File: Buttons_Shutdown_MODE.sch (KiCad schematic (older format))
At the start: 7 parts

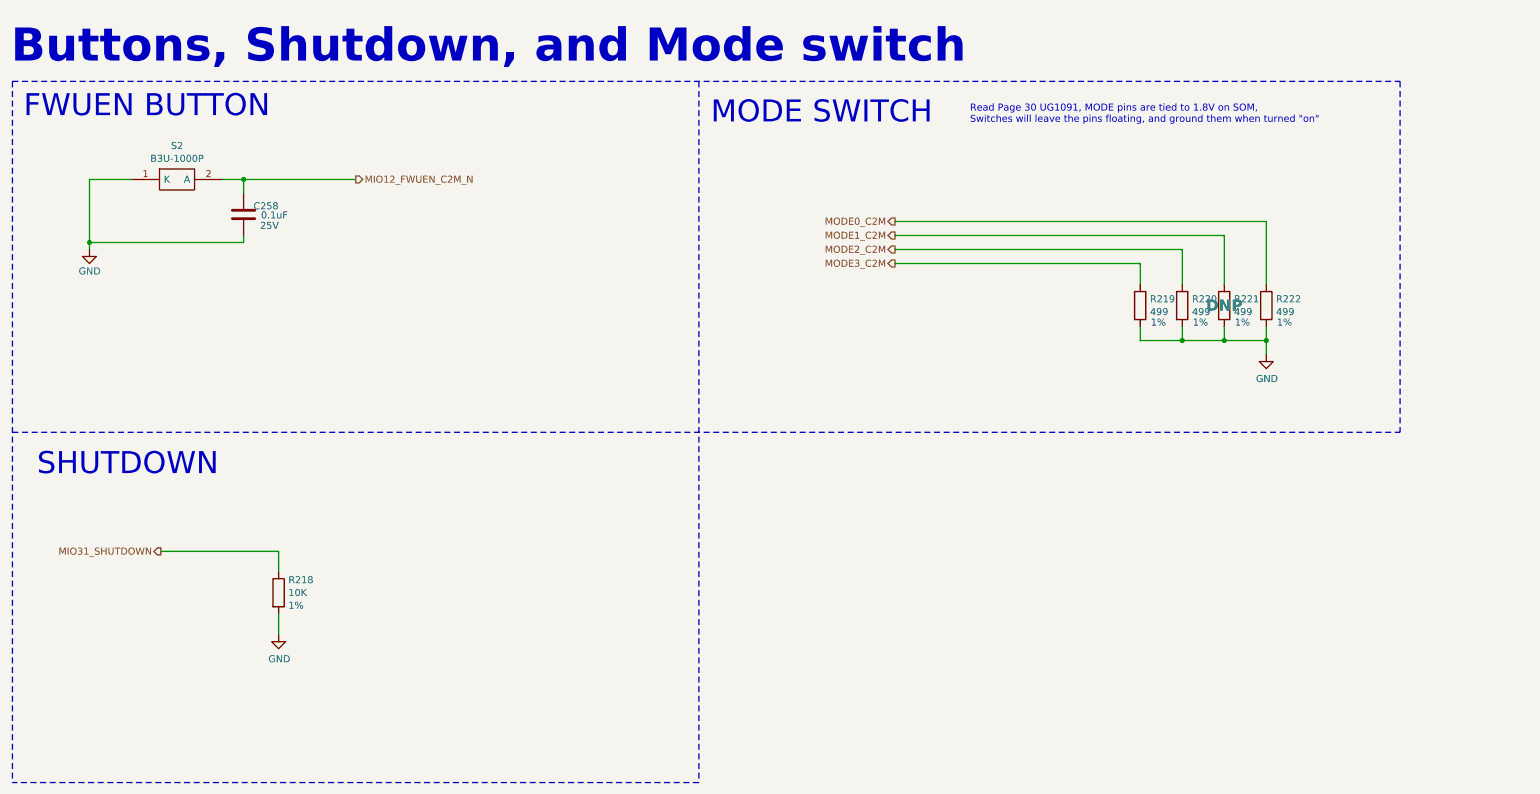
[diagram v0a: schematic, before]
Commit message: Update May --> See Update Note
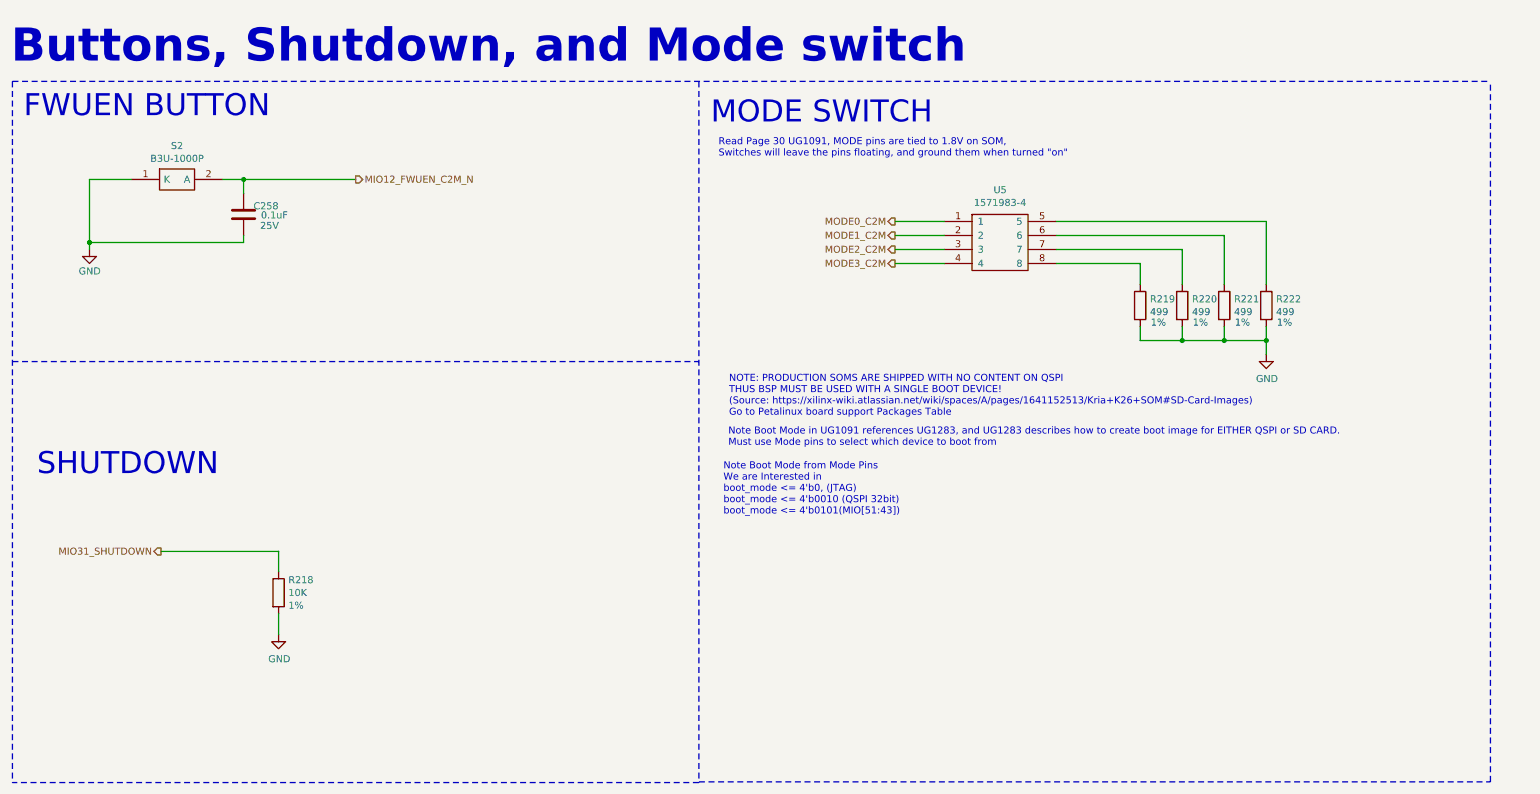
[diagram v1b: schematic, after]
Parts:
- added U5: 1571983-4, ApotheoTech_CXP_Lib:1571983-4, symbol ApotheoTech:1571983-4
- R221: DNP DNP -> (none)
- S2: footprint B3U-1000P -> ApotheoTech_CXP_Lib:B3U-1000P
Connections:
- net MODE0_C2M: now also U5.1; no longer R222.1
- net MODE1_C2M: now also U5.2; no longer R221.1
- net MODE2_C2M: now also U5.3; no longer R220.1
- net MODE3_C2M: now also U5.4; no longer R219.1
- new net: R219.1, U5.8
- new net: R220.1, U5.7
- new net: R221.1, U5.6
- new net: R222.1, U5.5
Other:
- note added: "NOTE: PRODUCTION SOMS ARE SHIPPED WITH NO CONTENT ON QSPI\nTHUS BSP MUST BE USED WITH A SINGLE BOOT DEVICE! \n(Source: https://xilinx-wiki.atlassian.net/wiki/spaces/A/pages/1641152513/Kria+K26+SOM#SD-Card-Images)\nGo to Petalinux board support Packages Table"
- note added: "Note Boot Mode from Mode Pins\nWe are Interested in \nboot_mode <= 4'b0, (JTAG)\nboot_mode <= 4'b0010 (QSPI 32bit)\nboot_mode <= 4'b0101(MIO[51:43])\n"
- note added: "Note Boot Mode in UG1091 references UG1283, and UG1283 describes how to create boot image for EITHER QSPI or SD CARD.\nMust use Mode pins to select which device to boot from\n"
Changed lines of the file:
@@
 F 0 "S2" H 1775 1940 50  0000 C CNN
 F 1 "B3U-1000P" H 1775 1849 50  0000 C CNN
-F 2 "B3U-1000P" H 2425 1800 50  0001 L CNN
+F 2 "ApotheoTech_CXP_Lib:B3U-1000P" H 2425 1800 50  0001 L CNN
 F 3 "https://www.omron.com/ecb/products/pdf/en-b3u.pdf" H 2425 1700 50  0001 L CNN
 F 4 "OMRON ELECTRONIC COMPONENTS - B3U-1000P - SWITCH, SPST-NO, 0.05A, 12V, SMD" H 2425 1600 50  0001 L CNN "Description"
@@
 Text HLabel 3050 1700 2    50   Output ~ 0
 MIO12_FWUEN_C2M_N
-Wire Notes Line
-	10505 1000 10505 3505
-Wire Notes Line
-	600  1000 10505 1000
-Wire Notes Line
-	600  3505 10505 3505
 Text Notes 5585 1315 0    157  ~ 0
 MODE SWITCH
 Text Notes 775  3825 0    157  ~ 0
 SHUTDOWN
-Text Notes 7435 1305 0    50   ~ 0
+Text Notes 5640 1545 0    50   ~ 0
 Read Page 30 UG1091, MODE pins are tied to 1.8V on SOM,\nSwitches will leave the pins floating, and ground them when turned "on"
 Text HLabel 6900 2000 0    50   Output ~ 0
@@
 F 5 "1%" H 9380 2480 50  0000 C CNN "Tol"
 F 6 "1/10W" H 9250 2600 50  0001 C CNN "Power"
-F 7 "DNP" H 9250 2600 79  0000 C CNB "DNP"
 	1    9250 2600
 	1    0    0    -1
@@
 Wire Notes Line
 	600  1000 600  6005
-Wire Wire Line
-	6900 2000 9550 2000
-Wire Wire Line
-	6900 2100 9250 2100
-Wire Wire Line
-	6900 2200 8950 2200
-Wire Wire Line
-	6900 2300 8650 2300
 $Comp
 L Device:R R?
@@
 	1    0    0    -1
 $EndComp
+Text Notes 5715 3395 0    50   ~ 0
+NOTE: PRODUCTION SOMS ARE SHIPPED WITH NO CONTENT ON QSPI\nTHUS BSP MUST BE USED WITH A SINGLE BOOT DEVICE! \n(Source: https://xilinx-wiki.atlassian.net/wiki/spaces/A/pages/1641152513/Kria+K26+SOM#SD-Card-Images)\nGo to Petalinux board support Packages Table
+Wire Notes Line
+	600  3000 5500 3000
+Text Notes 5710 3610 0    50   ~ 0
+Note Boot Mode in UG1091 references UG1283, and UG1283 describes how to create boot image for EITHER QSPI or SD CARD.\nMust use Mode pins to select which device to boot from\n
+Text Notes 5675 4100 0    50   ~ 0
+Note Boot Mode from Mode Pins\nWe are Interested in \nboot_mode <= 4'b0, (JTAG)\nboot_mode <= 4'b0010 (QSPI 32bit)\nboot_mode <= 4'b0101(MIO[51:43])\n
+$Comp
+L ApotheoTech:1571983-4 U5
+U 1 1 632384B2
+P 7650 2150
+F 0 "U5" H 7650 2525 50  0000 C CNN
+F 1 "1571983-4" H 7650 2434 50  0000 C CNN
+F 2 "ApotheoTech_CXP_Lib:1571983-4" H 7650 2150 50  0001 C CNN
+F 3 "" H 7650 2150 50  0001 C CNN
+	1    7650 2150
+	1    0    0    -1
+$EndComp
+Wire Wire Line
+	6900 2000 7250 2000
+Wire Wire Line
+	6900 2100 7250 2100
+Wire Wire Line
+	6900 2200 7250 2200
+Wire Wire Line
+	6900 2300 7250 2300
+Wire Wire Line
+	8050 2300 8650 2300
+Wire Wire Line
+	8050 2200 8950 2200
+Wire Wire Line
+	8050 2100 9250 2100
+Wire Wire Line
+	8050 2000 9550 2000
+Wire Notes Line
+	5500 6000 11150 6000
+Wire Notes Line
+	11150 6000 11150 1000
+Wire Notes Line
+	600  1000 11150 1000
 $EndSCHEMATC
